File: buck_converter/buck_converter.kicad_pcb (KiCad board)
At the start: 2 copper layers, 22 parts, among them Q1 IRF6641, U1 LM741, U2 LM741, U3 LM741, U4 LM741

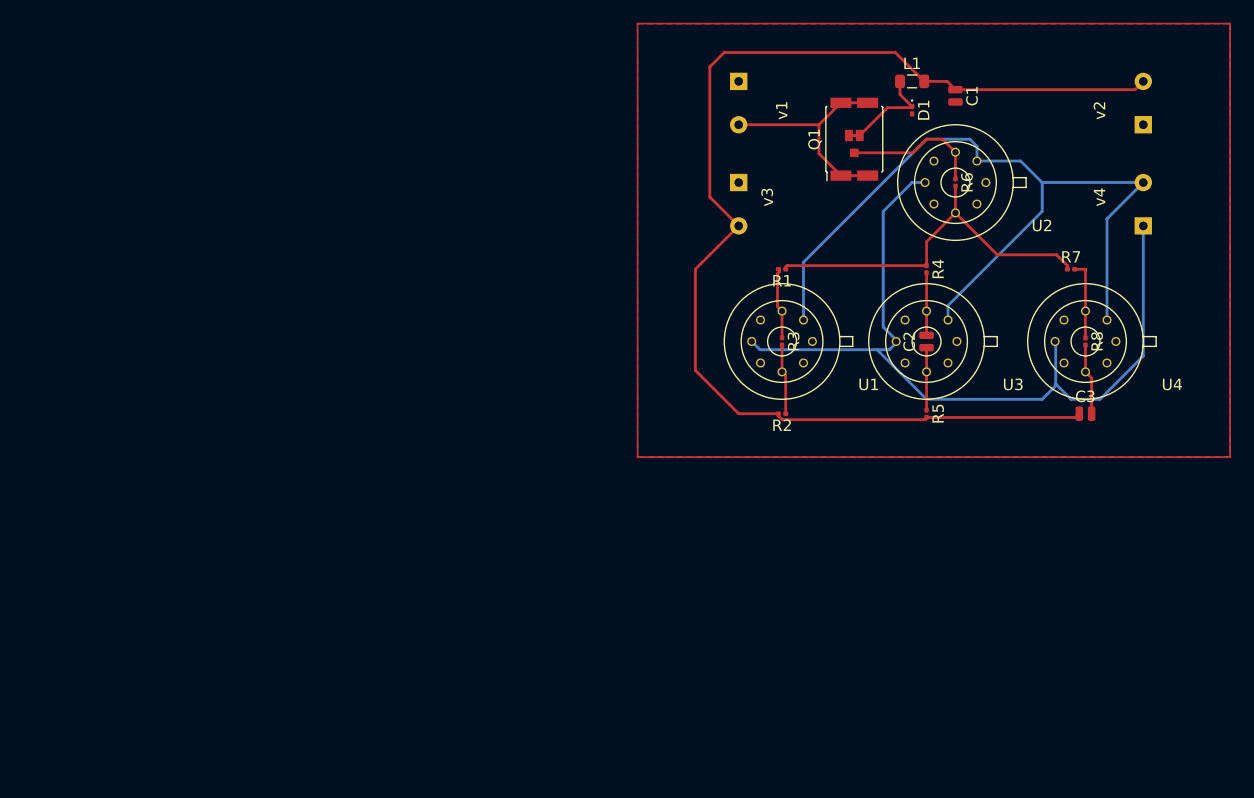
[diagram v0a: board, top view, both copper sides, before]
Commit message: güncelleme
kontrol edilmeyecek de olsa hatalı olduğumu belirttiğiniz noktaları düzeltmeye çalıştım
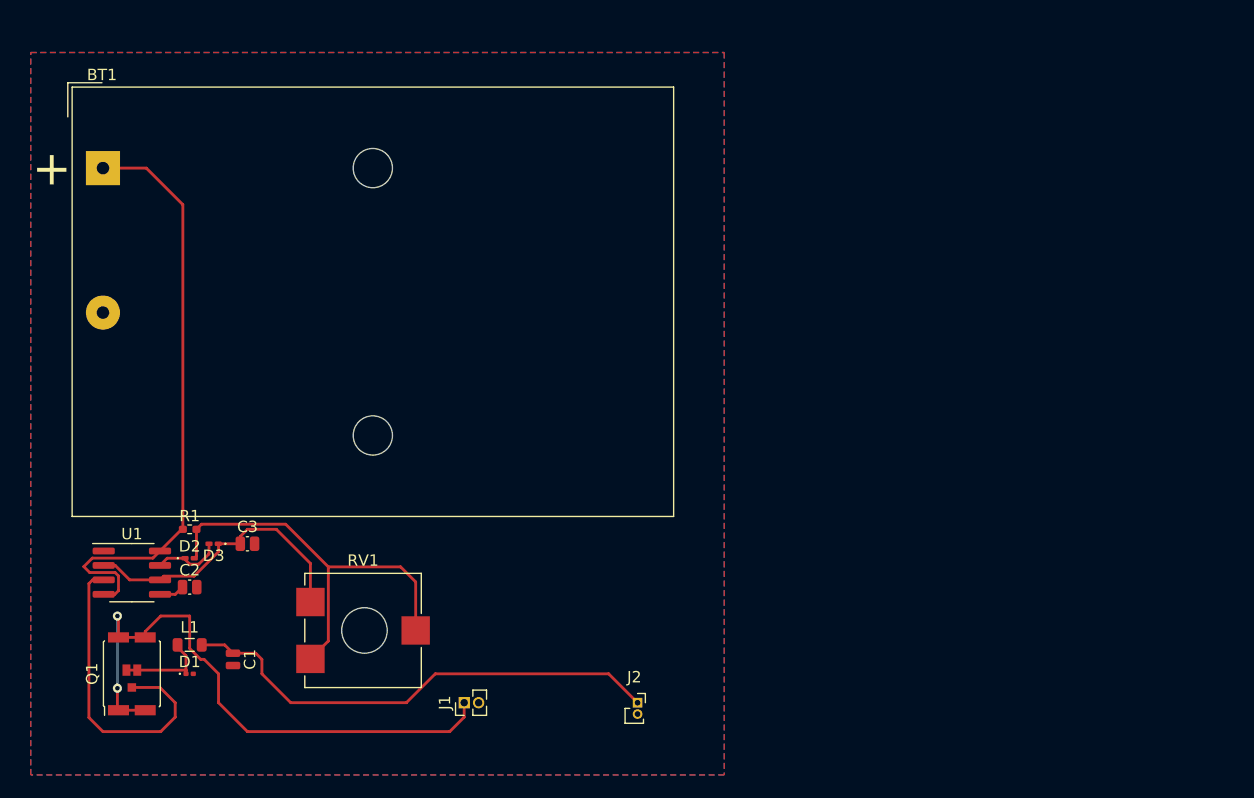
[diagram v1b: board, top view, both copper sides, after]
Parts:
- removed R2, R3, R4, R5, R6, R7, R8: R, Resistor_SMD:R_0201_0603Metric
- removed U2, U3, U4: LM741, opamp:lm741
- removed v1: vin, klemens:2xKlemens
- removed v2: load, klemens:2xKlemens
- removed v3: signal, klemens:2xKlemens
- removed v4: battery, klemens:2xKlemens
- added BT1: 4V5, Battery:BatteryHolder_Keystone_2479_3xAAA, F.Cu at (73.7, 80.0)
- added D2: D, Diode_SMD:D_0201_0603Metric_Pad0.64x0.40mm_HandSolder, F.Cu at (81.3, 114.3)
- added D3: D, Diode_SMD:D_0201_0603Metric_Pad0.64x0.40mm_HandSolder, F.Cu at (83.4, 113.0)
- added J1: Conn_01x02_Male, Connector_PinHeader_1.27mm:PinHeader_1x02_P1.27mm_Vertical, F.Cu at (105.4, 127.0)
- added J2: Conn_01x02_Female, Connector_PinSocket_1.00mm:PinSocket_1x02_P1.00mm_Vertical, F.Cu at (120.7, 127.0)
- added RV1: 100k, Potentiometer_SMD:Potentiometer_ACP_CA9-VSMD_Vertical_Hole, F.Cu at (96.5, 120.7)
- C1: value C -> 380uF
- C2: value C -> 10nF; footprint Capacitor_SMD:C_0504_1310Metric -> Capacitor_SMD:C_0504_1310Metric_Pad0.83x1.28mm_HandSolder
- C3: value C -> 1uF; footprint Capacitor_SMD:C_0504_1310Metric -> Capacitor_SMD:C_0504_1310Metric_Pad0.83x1.28mm_HandSolder
- L1: value INDUCTOR -> 100uH
- R1: value R -> 1k; footprint Resistor_SMD:R_0201_0603Metric -> Resistor_SMD:R_0402_1005Metric_Pad0.72x0.64mm_HandSolder
- U1: value LM741 -> NE555D; footprint opamp:lm741 -> Package_SO:SOIC-8_3.9x4.9mm_P1.27mm
- moved C1 80.5 mm to (85.1, 123.2)
- moved D1 80.5 mm to (81.3, 124.5), turned to 0 degrees
- moved L1 80.5 mm to (81.3, 121.9)
- moved Q1 79.0 mm to (76.2, 124.5)
- moved C3 74.5 mm to (86.4, 113.0)
- moved C2 68.3 mm to (81.3, 116.8), turned to 0 degrees
- moved U1 60.7 mm to (76.2, 115.6), turned to 0 degrees
- moved R1 56.9 mm to (81.3, 111.8), turned to 0 degrees
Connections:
- C2 pad 2: Net-(C2-Pad2) -> GNDREF
- C3 pad 1: Net-(C1-Pad1) -> Net-(C3-Pad1)
- C3 pad 2: Net-(C3-Pad2) -> GNDREF
- Q1 pad 2: Net-(Q1-Pad2) -> Signal
- R1 pad 1: Net-(R1-Pad1) -> Net-(BT1-Pad1)
- R1 pad 2: Net-(R1-Pad2) -> Net-(D2-Pad2)
- U1 pad 1: Net-(U1-Pad1) -> GNDREF
- U1 pad 2: Net-(R2-Pad1) -> Net-(C3-Pad1)
- U1 pad 3: GNDREF -> Signal
- U1 pad 4: -15V -> Net-(BT1-Pad1)
- U1 pad 5: Net-(U1-Pad5) -> Net-(C2-Pad1)
- U1 pad 6: Net-(R1-Pad2) -> Net-(C3-Pad1)
- U1 pad 7: +15V -> Net-(D2-Pad1)
- U1 pad 8: Net-(U1-Pad8) -> Net-(BT1-Pad1)
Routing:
- net -15V: track 73.2 -> 0.00 mm
- net +15V: track 70.7 -> 0.00 mm
- net Net-(C1-Pad1): track 105.5 -> 43.3 mm
- net Net-(BT1-Pad1): track 0.00 -> 53.1 mm
- net Net-(D2-Pad2): track 0.00 -> 37.4 mm
- net Net-(J1-Pad1): track 19.8 -> 53.2 mm, vias 0 -> 2
- net Net-(R1-Pad1): track 32.7 -> 0.00 mm
- net Signal: track 0.00 -> 27.6 mm
- net Net-(C3-Pad1): track 0.00 -> 27.0 mm
- net Net-(Q1-Pad2): track 12.2 -> 0.00 mm
- net Net-(R7-Pad2): track 6.98 -> 0.00 mm
- net Net-(R1-Pad2): track 6.30 -> 0.00 mm
- net Net-(C3-Pad2): track 6.25 -> 0.00 mm
- net Net-(R2-Pad1): track 6.16 -> 0.00 mm
- net Net-(D2-Pad1): track 0.00 -> 6.11 mm
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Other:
- board text added: "DC-DC Buck Converter"
- board text added: "RND Electronic"
